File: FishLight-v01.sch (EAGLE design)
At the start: 216 parts, among them Q1 RK7002BSOT23-3, Q10 RK7002BSOT23-3, Q11 RK7002BSOT23-3, Q12 RK7002BSOT23-3, Q13 RK7002BSOT23-3, Q14 RK7002BSOT23-3, Q15 RK7002BSOT23-3, Q2 RK7002BSOT23-3, Q3 RK7002BSOT23-3, Q4 RK7002BSOT23-3, Q5 RK7002BSOT23-3, Q6 RK7002BSOT23-3, Q7 RK7002BSOT23-3, Q8 RK7002BSOT23-3, Q9 RK7002BSOT23-3, U1 SPARK_CORECORE, U10 AD5248MSOP-10, U11 INA219SOT23-8, U12 INA219SOT23-8, U13 INA219SOT23-8, U14 INA219SOT23-8, U15 INA219SOT23-8, U16 MIC29300D2PAK-3, U17 L7805D2PAK-2, U2 DS3231MSOIC-8, U22 AD5248MSOP-10, U23 CAT4101TO-263, U24 CAT4101TO-263, U25 CAT4101TO-263, U26 INA219SOT23-8, U27 INA219SOT23-8, U28 INA219SOT23-8, U29 CD74HC4067SSOP24, U3 CAT4101TO-263, U30 CD74HC4067SSOP24, U31 RELAY-SOLIDSTATEPTH, U32 RELAY-SOLIDSTATEPTH, U33 RELAY-SOLIDSTATEPTH, U34 NC7SZ373TSSOP-6, U35 NC7SZ373TSSOP-6, U36 NC7SZ373TSSOP-6, U37 NC7SZ373TSSOP-6, U38 NC7SZ373TSSOP-6, U39 NC7SZ373TSSOP-6, U4 CAT4101TO-263, U40 NC7SZ373TSSOP-6, U41 NC7SZ373TSSOP-6, U42 NC7SZ373TSSOP-6, U43 NC7SZ373TSSOP-6, U44 NC7SZ373TSSOP-6, U45 NC7SZ373TSSOP-6, U46 NC7SZ373TSSOP-6, U47 NC7SZ373TSSOP-6, U48 NC7SZ373TSSOP-6, U49 DS18B20USOP8, U5 CAT4101TO-263, U6 CAT4101TO-263, U7 CAT4101TO-263, U8 AD5248MSOP-10, U9 AD5248MSOP-10

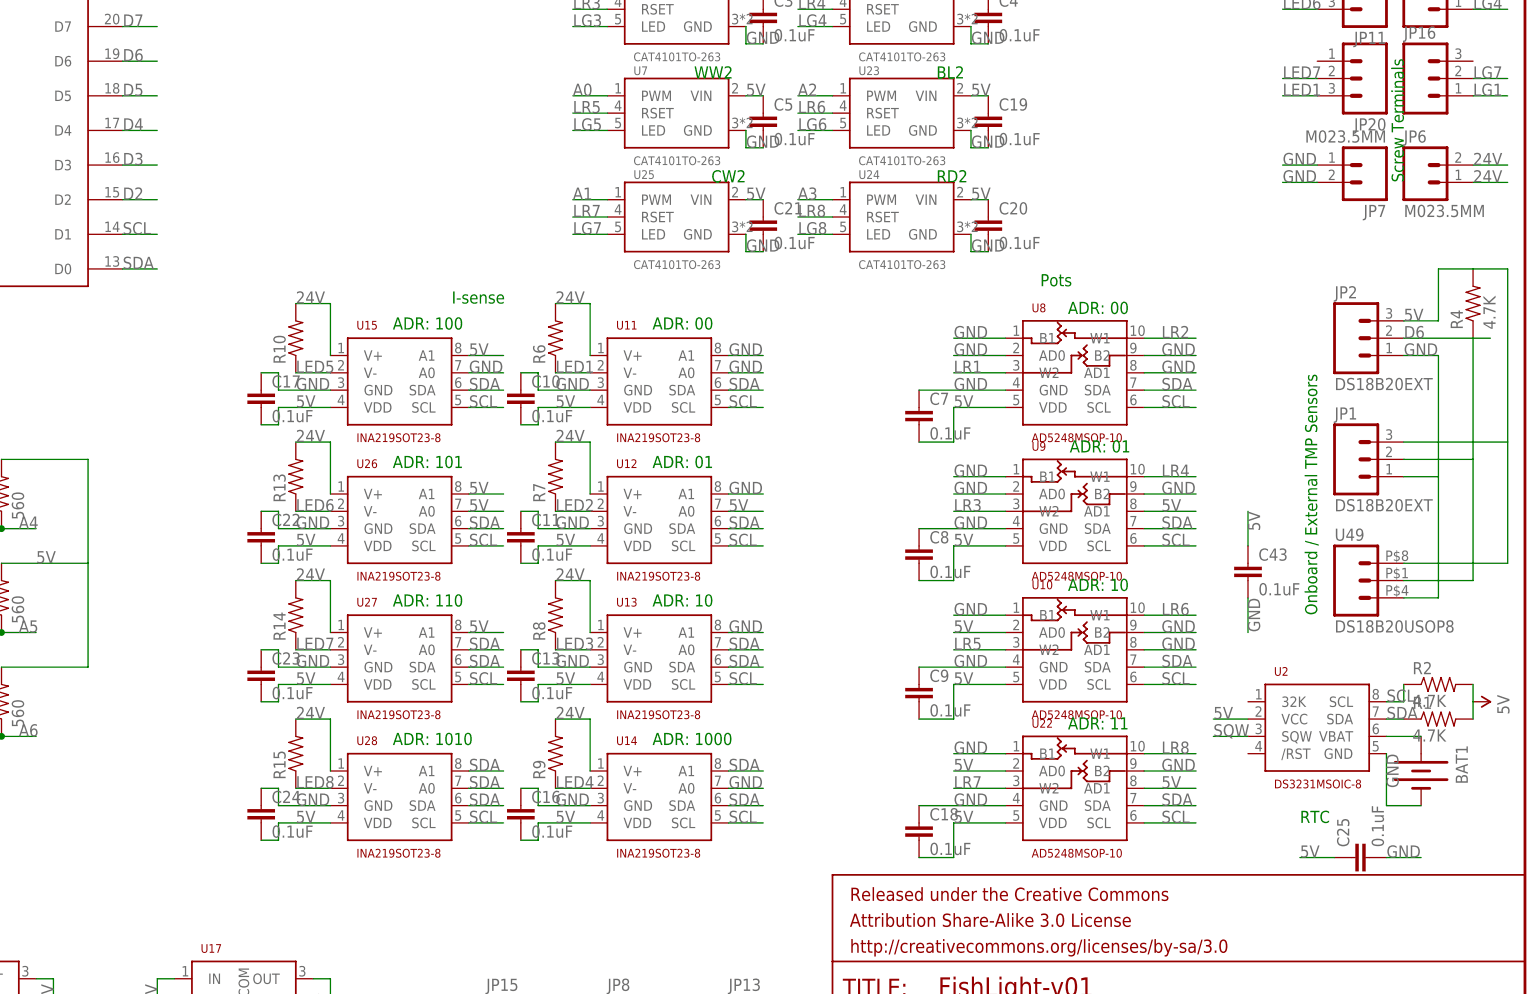
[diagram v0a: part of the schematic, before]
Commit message: FishLight_PCB: Remove the RTC
The RTC isn't really needed because the Spark Core can get the time
directly from the internet and it has an onboard RTC that can be used
instead.  The only downside is that it doesn't have a battery but it can
just sync with the internet at startup.  It also has EEPROM like memory
that can be accessed to store data as needed, just like an RTC would
have.
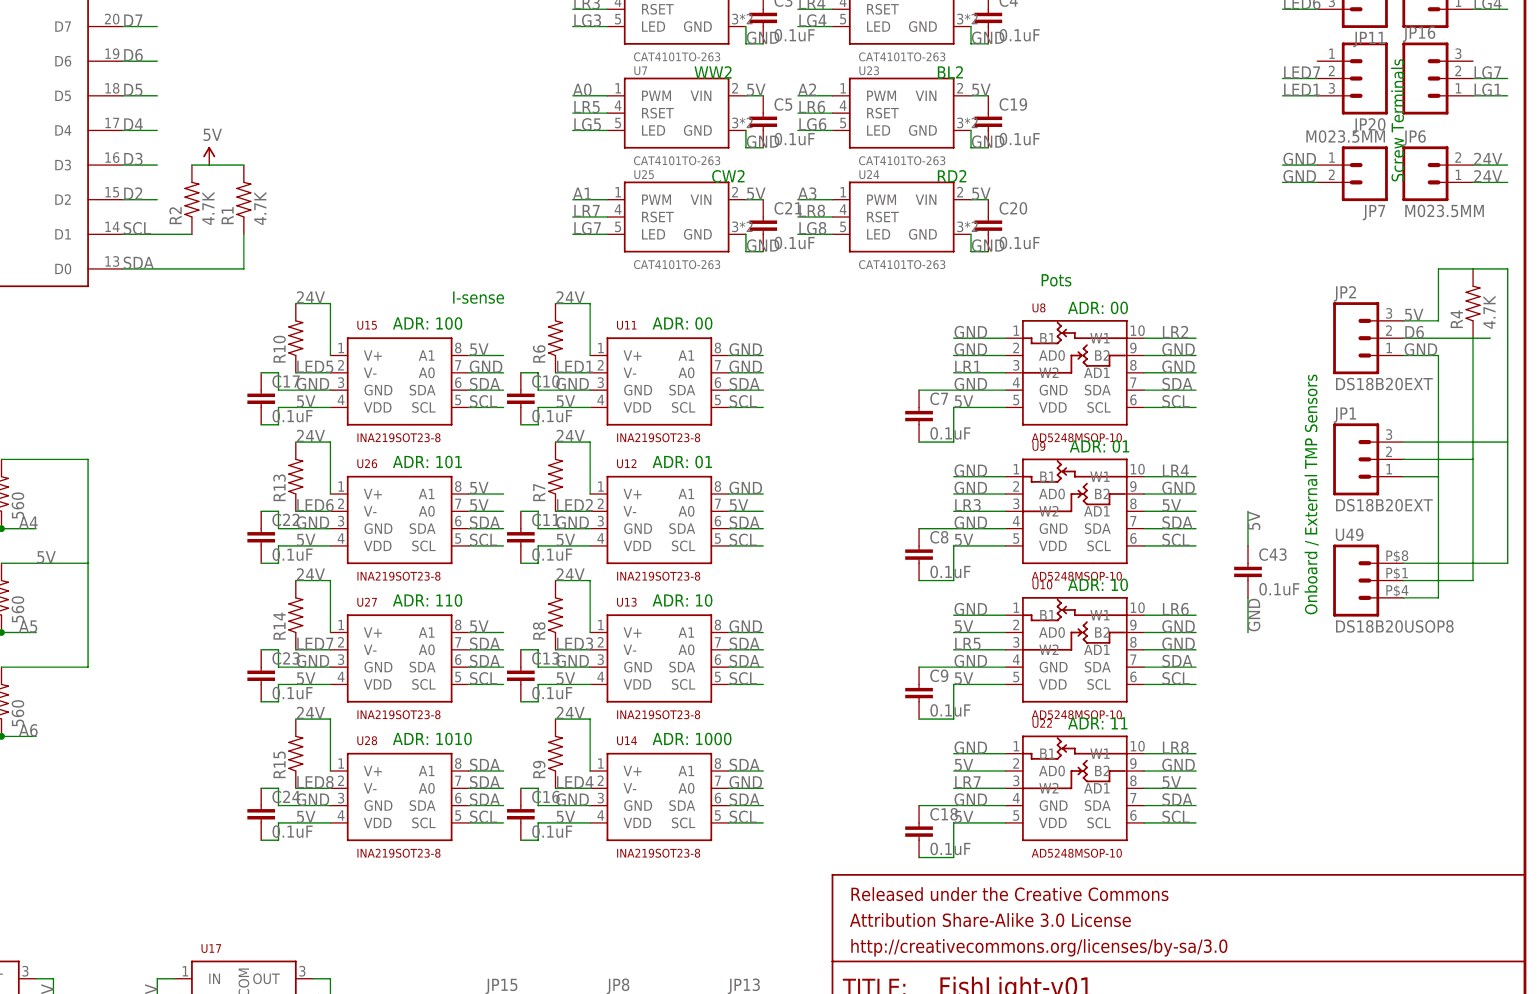
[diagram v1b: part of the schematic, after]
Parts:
- removed BAT1: (no value), SparkFun-Electromechanical:BATTERY12PTH
- removed C25: 0.1uF, SparkFun-Capacitors:0.1UF-25V(+80/-20%)(0603)
- removed U2: DS3231MSOIC-8, Mikes-Stuff:DS3231MSOIC-8
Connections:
- removed net N$3: BAT1.+, U2.VBAT
- removed net SQW: U2.SQW
- net 5V: no longer C25.1, U2.VCC
- net GND: no longer BAT1.-, C25.2, U2.GND
- net SCL: no longer U2.SCL
- net SDA: no longer U2.SDA
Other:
- note removed: "RTC"
- moved on the sheet: R1, R2
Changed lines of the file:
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@@
 <part name="C23" library="SparkFun-Capacitors" deviceset="0.1UF-25V(+80/-20%)(0603)" device="" value="0.1uF"/>
 <part name="C24" library="SparkFun-Capacitors" deviceset="0.1UF-25V(+80/-20%)(0603)" device="" value="0.1uF"/>
-<part name="U2" library="Mikes-Stuff" deviceset="DS3231M" device="SOIC-8"/>
-<part name="BAT1" library="SparkFun-Electromechanical" deviceset="BATTERY" device="12PTH"/>
-<part name="C25" library="SparkFun-Capacitors" deviceset="0.1UF-25V(+80/-20%)(0603)" device="" value="0.1uF"/>
 <part name="JP17" library="Mikes-Stuff" deviceset="M02" device="2.54MM_SCREWTERM"/>
 <part name="JP19" library="Mikes-Stuff" deviceset="M02" device="2.54MM_SCREWTERM"/>
@@
 <text x="91.44" y="-20.32" size="1.778" layer="91">LED: 2.2V, 20mA</text>
 <text x="5.08" y="55.88" size="1.778" layer="91" rot="R90">Water Level Sensors</text>
-<text x="215.9" y="43.18" size="1.778" layer="91">RTC</text>
 <text x="177.8" y="121.92" size="1.778" layer="91">Pots</text>
 </plain>
@@
 <instance part="C4" gate="G$1" x="170.18" y="160.02"/>
 <instance part="C5" gate="G$1" x="137.16" y="144.78"/>
-<instance part="R1" gate="G$1" x="236.22" y="58.42"/>
-<instance part="R2" gate="G$1" x="236.22" y="63.5"/>
-<instance part="5V1" gate="G$1" x="241.3" y="60.96" rot="R270"/>
+<instance part="R1" gate="G$1" x="60.96" y="134.62" rot="R90"/>
+<instance part="R2" gate="G$1" x="53.34" y="134.62" rot="R90"/>
+<instance part="5V1" gate="G$1" x="55.88" y="139.7"/>
 <instance part="C7" gate="G$1" x="160.02" y="101.6"/>
 <instance part="C8" gate="G$1" x="160.02" y="81.28"/>
@@
 <instance part="C23" gate="G$1" x="63.5" y="63.5"/>
 <instance part="C24" gate="G$1" x="63.5" y="43.18"/>
-<instance part="U2" gate="G$1" x="218.44" y="58.42"/>
-<instance part="BAT1" gate="G$1" x="233.68" y="50.8" rot="R270"/>
-<instance part="C25" gate="G$1" x="226.06" y="38.1" rot="R90"/>
 <instance part="JP17" gate="G$1" x="38.1" y="-144.78"/>
 <instance part="JP19" gate="G$1" x="30.48" y="-142.24" rot="R180"/>
@@
 <net name="SDA" class="0">
 <segment>
-<wire x1="228.6" y1="58.42" x2="231.14" y2="58.42" width="0.1524" layer="91"/>
-<label x="228.6" y="58.42" size="1.778" layer="95"/>
-<pinref part="R1" gate="G$1" pin="1"/>
-<pinref part="U2" gate="G$1" pin="SDA"/>
-</segment>
-<segment>
 <pinref part="JP18" gate="G$1" pin="2"/>
 <wire x1="12.7" y1="109.22" x2="17.78" y2="109.22" width="0.2032" layer="91"/>
@@
 <segment>
 <pinref part="U1" gate="G$1" pin="D0"/>
-<wire x1="43.18" y1="124.46" x2="48.26" y2="124.46" width="0.2032" layer="91"/>
 <label x="43.18" y="124.46" size="1.778" layer="95"/>
+<pinref part="R1" gate="G$1" pin="1"/>
+<wire x1="43.18" y1="124.46" x2="60.96" y2="124.46" width="0.2032" layer="91"/>
+<wire x1="60.96" y1="124.46" x2="60.96" y2="129.54" width="0.2032" layer="91"/>
 </segment>
 <segment>
@@
 <net name="SCL" class="0">
 <segment>
-<wire x1="228.6" y1="60.96" x2="231.14" y2="60.96" width="0.1524" layer="91"/>
-<label x="228.6" y="60.96" size="1.778" layer="95"/>
-<pinref part="R2" gate="G$1" pin="1"/>
-<wire x1="231.14" y1="63.5" x2="231.14" y2="60.96" width="0.2032" layer="91"/>
-<pinref part="U2" gate="G$1" pin="SCL"/>
-</segment>
-<segment>
 <wire x1="200.66" y1="63.5" x2="193.04" y2="63.5" width="0.2032" layer="91"/>
 <label x="195.58" y="63.5" size="1.778" layer="95"/>
@@
 <segment>
 <pinref part="U1" gate="G$1" pin="D1"/>
-<wire x1="43.18" y1="129.54" x2="48.26" y2="129.54" width="0.2032" layer="91"/>
 <label x="43.18" y="129.54" size="1.778" layer="95"/>
+<pinref part="R2" gate="G$1" pin="1"/>
+<wire x1="43.18" y1="129.54" x2="53.34" y2="129.54" width="0.2032" layer="91"/>
 </segment>
 </net>
@@
 <label x="2.54" y="175.26" size="1.778" layer="91"/>
 <pinref part="U1" gate="G$1" pin="GND@2"/>
-</segment>
-<segment>
-<label x="228.6" y="53.34" size="1.778" layer="95" rot="R270"/>
-<pinref part="BAT1" gate="G$1" pin="-"/>
-<wire x1="233.68" y1="45.72" x2="228.6" y2="45.72" width="0.2032" layer="91"/>
-<wire x1="228.6" y1="45.72" x2="228.6" y2="53.34" width="0.2032" layer="91"/>
-<pinref part="U2" gate="G$1" pin="GND"/>
 </segment>
 <segment>
@@
 <pinref part="C10" gate="G$1" pin="1"/>
 <label x="106.68" y="106.68" size="1.778" layer="95"/>
-</segment>
-<segment>
-<pinref part="C25" gate="G$1" pin="2"/>
-<wire x1="228.6" y1="38.1" x2="233.68" y2="38.1" width="0.2032" layer="91"/>
-<label x="228.6" y="38.1" size="1.778" layer="95"/>
 </segment>
 <segment>
@@
 <net name="5V" class="0">
 <segment>
-<wire x1="203.2" y1="58.42" x2="208.28" y2="58.42" width="0.1524" layer="91"/>
-<label x="203.2" y="58.42" size="1.778" layer="95"/>
-<pinref part="U2" gate="G$1" pin="VCC"/>
-</segment>
-<segment>
 <pinref part="U3" gate="G$1" pin="VIN"/>
 <pinref part="C1" gate="G$1" pin="1"/>
@@
 <wire x1="93.98" y1="71.12" x2="99.06" y2="71.12" width="0.2032" layer="91"/>
 <label x="93.98" y="71.12" size="1.778" layer="95"/>
-</segment>
-<segment>
-<pinref part="R2" gate="G$1" pin="2"/>
-<pinref part="5V1" gate="G$1" pin="5V"/>
-<pinref part="R1" gate="G$1" pin="2"/>
-<wire x1="241.3" y1="63.5" x2="241.3" y2="60.96" width="0.2032" layer="91"/>
-<wire x1="241.3" y1="60.96" x2="241.3" y2="58.42" width="0.2032" layer="91"/>
-</segment>
-<segment>
-<pinref part="C25" gate="G$1" pin="1"/>
-<wire x1="220.98" y1="38.1" x2="215.9" y2="38.1" width="0.2032" layer="91"/>
-<label x="215.9" y="38.1" size="1.778" layer="95"/>
 </segment>
 <segment>
@@
 <label x="208.28" y="88.9" size="1.778" layer="95" rot="R270"/>
 </segment>
-</net>
-<net name="SQW" class="0">
-<segment>
-<wire x1="208.28" y1="55.88" x2="203.2" y2="55.88" width="0.1524" layer="91"/>
-<label x="203.2" y="55.88" size="1.778" layer="95"/>
-<pinref part="U2" gate="G$1" pin="SQW"/>
+<segment>
+<pinref part="R2" gate="G$1" pin="2"/>
+<pinref part="5V1" gate="G$1" pin="5V"/>
+<wire x1="53.34" y1="139.7" x2="55.88" y2="139.7" width="0.2032" layer="91"/>
+<pinref part="R1" gate="G$1" pin="2"/>
+<wire x1="60.96" y1="139.7" x2="55.88" y2="139.7" width="0.2032" layer="91"/>
 </segment>
 </net>
@@
 </segment>
 </net>
-<net name="N$3" class="0">
-<segment>
-<pinref part="U2" gate="G$1" pin="VBAT"/>
-<pinref part="BAT1" gate="G$1" pin="+"/>
-<wire x1="228.6" y1="55.88" x2="233.68" y2="55.88" width="0.2032" layer="91"/>
-</segment>
-</net>
